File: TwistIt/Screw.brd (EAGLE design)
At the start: 33.5 x 36.5 mm, 8 parts

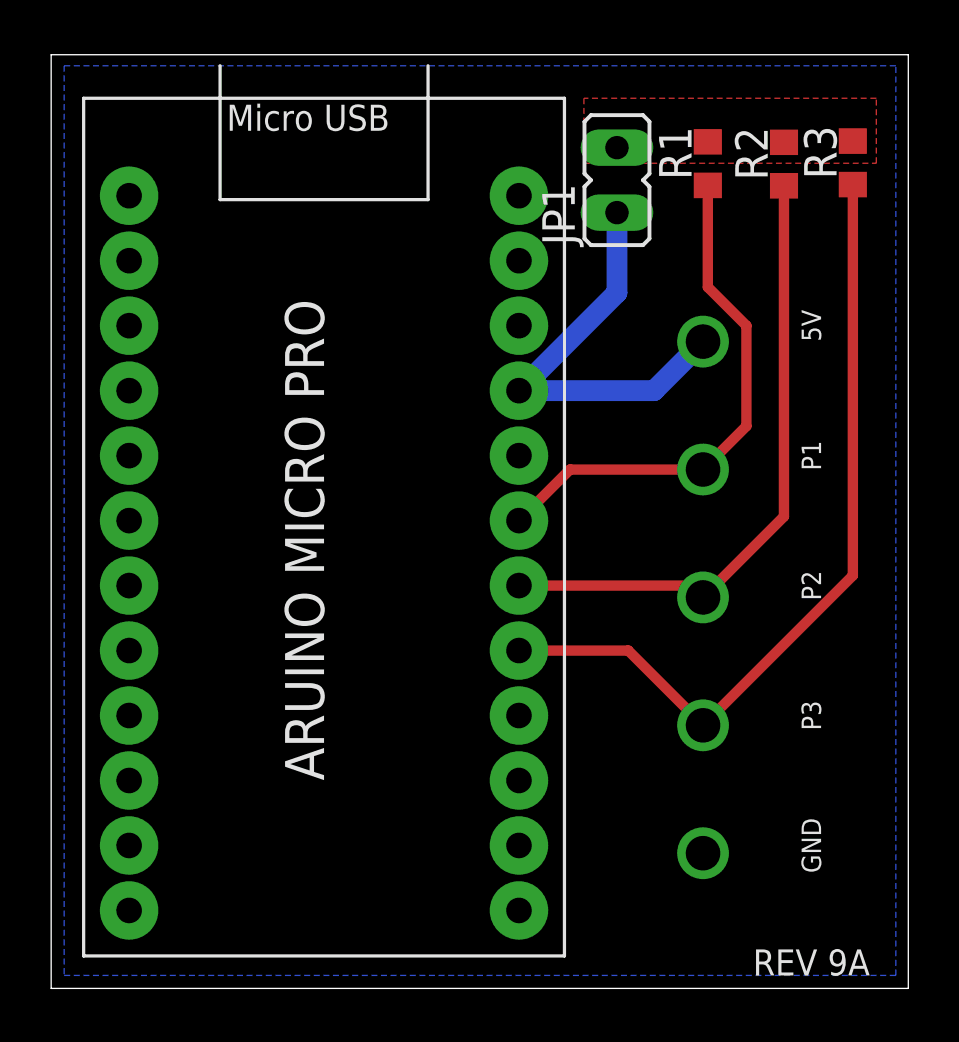
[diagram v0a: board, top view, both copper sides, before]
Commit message: Minor fixes everywhere
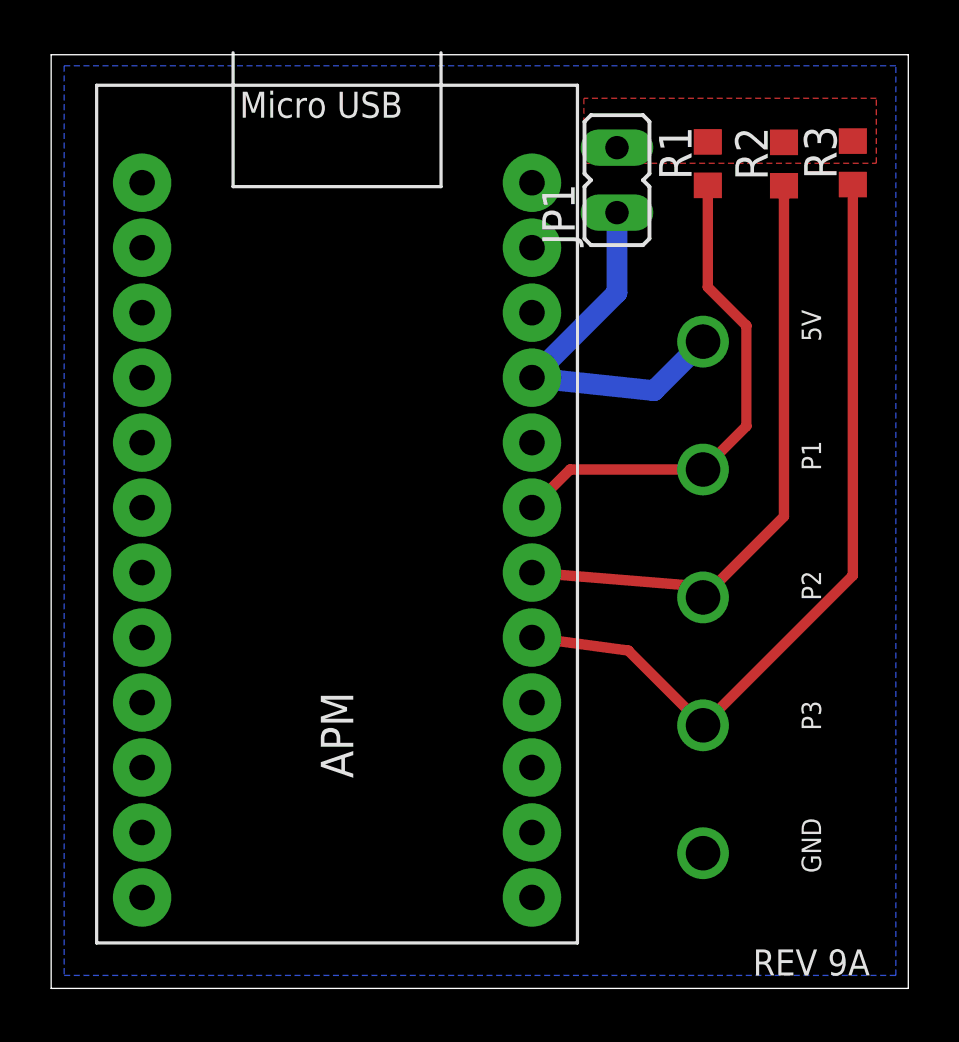
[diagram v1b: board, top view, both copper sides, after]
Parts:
- R1, R2, R3: value (none) -> 330
- ST1: value 5PIN_SCREW -> (none)
- renumbered U$1 to APM, U$2 to ST1
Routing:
- net VCC: track 16.5 -> 15.3 mm
- net P1: track 20.5 -> 19.7 mm
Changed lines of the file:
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@@
 <elements>
 <element name="JP1" library="jumper" package="JP1" value="" x="22.11928125" y="31.597309375"/>
-<element name="R1" library="resistor" package="R0603" value="" x="25.66984375" y="32.243665625" rot="R90"/>
-<element name="R2" library="resistor" package="R0603" value="" x="28.647703125" y="32.22621875" rot="R90"/>
-<element name="R3" library="resistor" package="R0603" value="" x="31.33979375" y="32.273709375" rot="R90"/>
-<element name="U$1" library="pie" package="ARDUINO_PRO_MICRO" value="ARDUINO_PRO_MICRO" x="1.778" y="1.778"/>
-<element name="U$2" library="pie" package="5PIN_SCREW" value="5PIN_SCREW" x="28.783865625" y="28.3851625" rot="MR270"/>
+<element name="R1" library="resistor" package="R0603" value="330" x="25.66984375" y="32.243665625" rot="R90"/>
+<element name="R2" library="resistor" package="R0603" value="330" x="28.647703125" y="32.22621875" rot="R90"/>
+<element name="R3" library="resistor" package="R0603" value="330" x="31.33979375" y="32.273709375" rot="R90"/>
+<element name="APM" library="pie" package="ARDUINO_PRO_MICRO" value="ARDUINO_PRO_MICRO" x="1.778" y="1.778"/>
+<element name="ST1" library="pie" package="5PIN_SCREW" value="" x="28.783865625" y="28.3851625" rot="MR270"/>
 <element name="U$3" library="pie" package="PIE-LOGO-SMALL" value="" x="5.842" y="27.94" rot="MR0"/>
 <element name="U$4" library="pie" package="OSHW-LOGO-S" value="" x="3.302" y="33.782" rot="MR0"/>
@@
 </signal>
 <signal name="GND">
-<contactref element="U$1" pad="GND@0"/>
+<contactref element="APM" pad="GND@0"/>
 <polygon width="0.4064" layer="16">
 <vertex x="0.508" y="36.068"/>
@@
 <vertex x="33.02" y="36.068"/>
 </polygon>
-<contactref element="U$2" pad="P$5"/>
+<contactref element="ST1" pad="P$5"/>
 </signal>
 <signal name="VCC">
-<contactref element="U$2" pad="P$1"/>
+<contactref element="ST1" pad="P$1"/>
 <contactref element="JP1" pad="1"/>
-<contactref element="U$1" pad="VCC"/>
-<wire x1="18.288" y1="23.368" x2="22.11928125" y2="27.19928125" width="0.8128" layer="16"/>
+<contactref element="APM" pad="VCC"/>
+<wire x1="18.796" y1="23.876" x2="22.11928125" y2="27.19928125" width="0.8128" layer="16"/>
 <wire x1="22.11928125" y1="27.19928125" x2="22.11928125" y2="30.327309375" width="0.8128" layer="16"/>
 <wire x1="25.483865625" y1="25.2851625" x2="23.566703125" y2="23.368" width="0.8128" layer="16"/>
-<wire x1="23.566703125" y1="23.368" x2="18.288" y2="23.368" width="0.8128" layer="16"/>
+<wire x1="23.566703125" y1="23.368" x2="18.796" y2="23.876" width="0.8128" layer="16"/>
 </signal>
 <signal name="P1">
 <contactref element="R1" pad="1"/>
-<contactref element="U$2" pad="P$2"/>
-<contactref element="U$1" pad="A2"/>
-<wire x1="18.288" y1="18.288" x2="20.2851625" y2="20.2851625" width="0.4064" layer="1"/>
+<contactref element="ST1" pad="P$2"/>
+<contactref element="APM" pad="A2"/>
+<wire x1="18.796" y1="18.796" x2="20.2851625" y2="20.2851625" width="0.4064" layer="1"/>
 <wire x1="20.2851625" y1="20.2851625" x2="25.483865625" y2="20.2851625" width="0.4064" layer="1"/>
 <wire x1="25.483865625" y1="20.2851625" x2="27.178" y2="21.979296875" width="0.4064" layer="1"/>
@@
 </signal>
 <signal name="P2">
-<contactref element="U$2" pad="P$3"/>
-<contactref element="U$1" pad="A1"/>
+<contactref element="ST1" pad="P$3"/>
+<contactref element="APM" pad="A1"/>
 <contactref element="R2" pad="1"/>
 <wire x1="25.483865625" y1="15.2851625" x2="28.647703125" y2="18.449" width="0.4064" layer="1"/>
 <wire x1="28.647703125" y1="18.449" x2="28.647703125" y2="31.37621875" width="0.4064" layer="1"/>
 <wire x1="25.483865625" y1="15.2851625" x2="25.021028125" y2="15.748" width="0.4064" layer="1"/>
-<wire x1="25.021028125" y1="15.748" x2="18.288" y2="15.748" width="0.4064" layer="1"/>
+<wire x1="25.021028125" y1="15.748" x2="18.796" y2="16.256" width="0.4064" layer="1"/>
 </signal>
 <signal name="P3">
-<contactref element="U$2" pad="P$4"/>
-<contactref element="U$1" pad="A0"/>
+<contactref element="ST1" pad="P$4"/>
+<contactref element="APM" pad="A0"/>
 <contactref element="R3" pad="1"/>
 <wire x1="25.483865625" y1="10.2851625" x2="22.561028125" y2="13.208" width="0.4064" layer="1"/>
-<wire x1="22.561028125" y1="13.208" x2="18.288" y2="13.208" width="0.4064" layer="1"/>
+<wire x1="22.561028125" y1="13.208" x2="18.796" y2="13.716" width="0.4064" layer="1"/>
 <wire x1="25.483865625" y1="10.2851625" x2="31.33979375" y2="16.141090625" width="0.4064" layer="1"/>
 <wire x1="31.33979375" y1="16.141090625" x2="31.33979375" y2="31.423709375" width="0.4064" layer="1"/>
